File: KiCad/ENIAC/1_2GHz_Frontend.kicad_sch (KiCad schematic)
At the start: 1 part, among them U12 HMC361S8GE

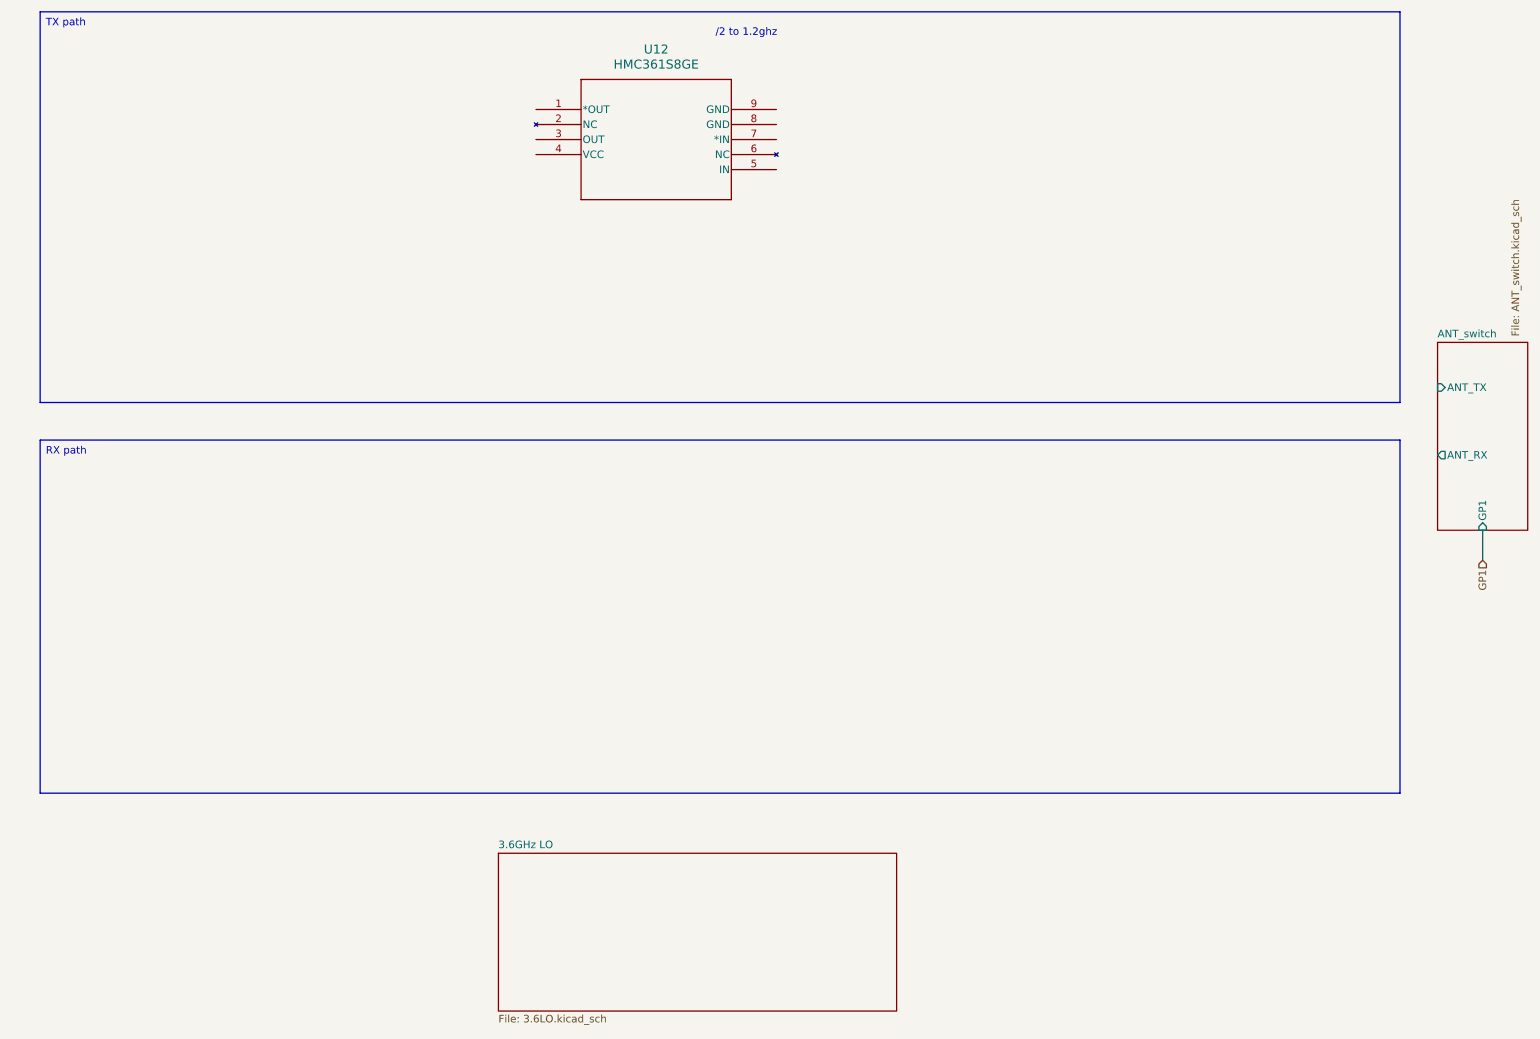
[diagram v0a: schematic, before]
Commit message: john d tickle
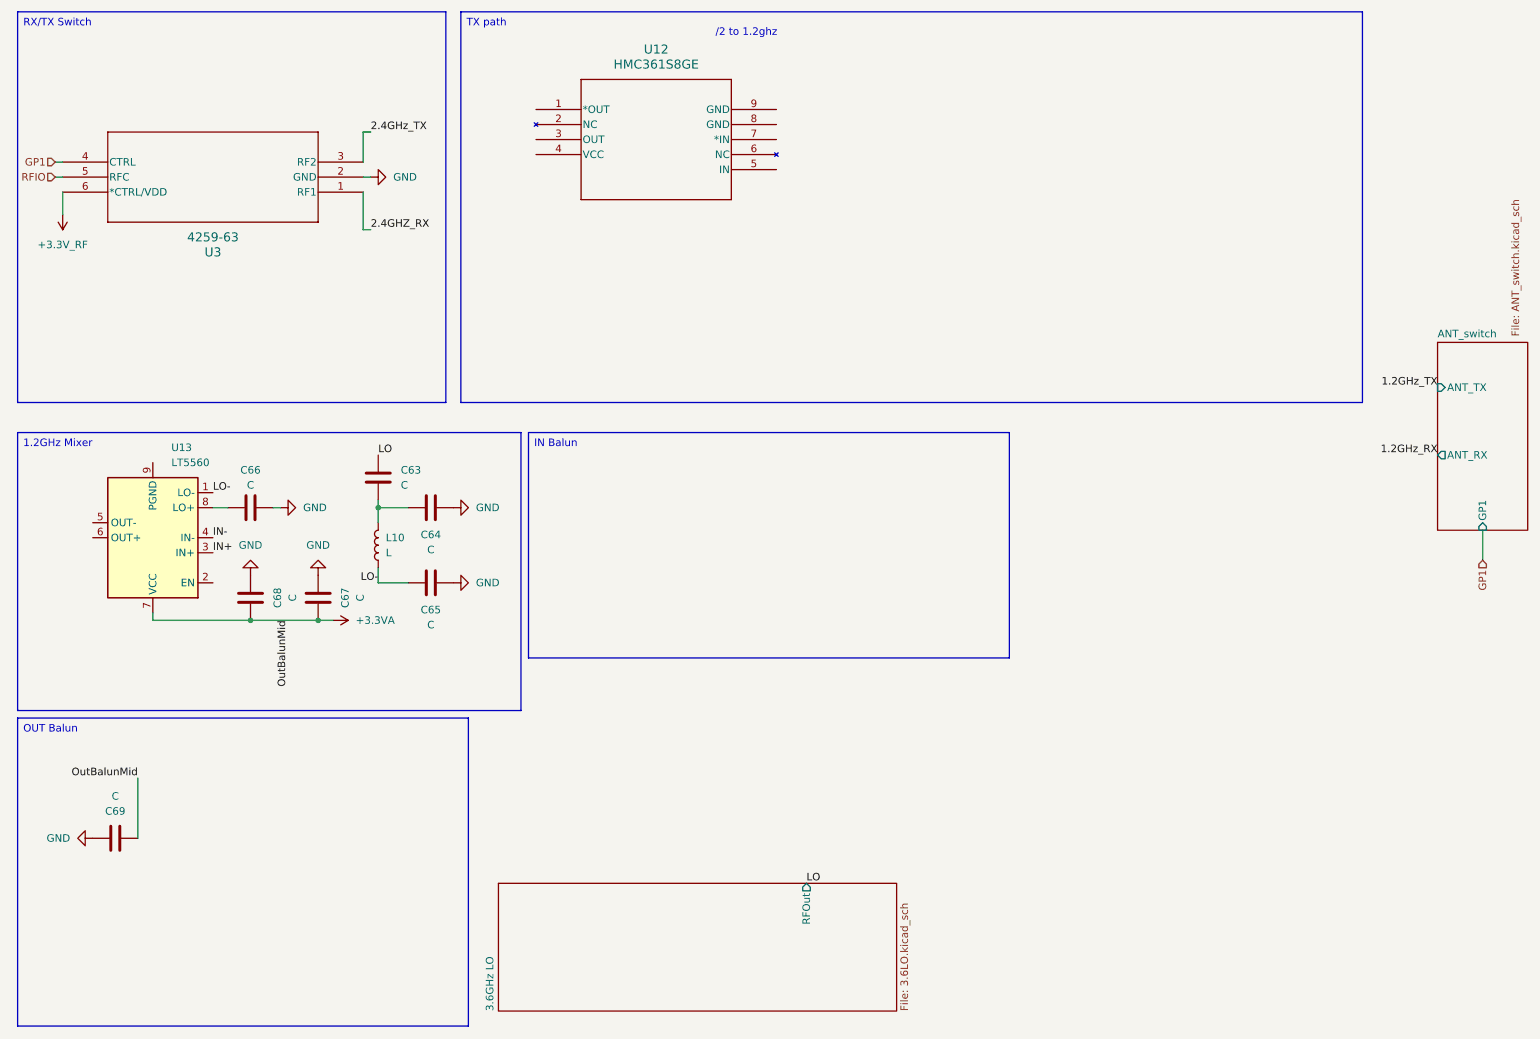
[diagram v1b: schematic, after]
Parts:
- added C63, C64, C65, C66, C67, C68, C69: C, symbol Device:C
- added L10: L, symbol Device:L
- added U13: LT5560, Package_DFN_QFN:DFN-8-1EP_3x3mm_P0.5mm_EP1.66x2.38mm, symbol RF_Mixer:LT5560
- added U3: 4259-63, SC-70-6_PSM, symbol 2025-11-10_00-05-56:4259-63
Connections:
- net GP1: now also U3.4 (CTRL)
- new net: C63.2, C64.1, L10.2
- new net: C66.1, U13.8 (LO+)
- new net +3.3VA: C67.1, C68.1, C69.1, U13.7 (VCC)
- new net +3.3V_RF: U3.6 (*CTRL/VDD)
- new net 2.4GHZ_RX: U3.1 (RF1)
- new net 2.4GHz_TX: U3.3 (RF2)
- new net GND: C64.2, C65.2, C66.2, C67.2, C68.2, C69.2, U3.2 (GND)
- new net IN+: U13.3 (IN+)
- new net IN-: U13.4 (IN-)
- new net LO: C63.1
- new net LO-: C65.1, L10.1, U13.1 (LO-)
- new net RFIO: U3.5 (RFC)
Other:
- sheet 3.6GHz LO ports: added RFOut; removed none
